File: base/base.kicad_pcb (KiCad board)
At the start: 2 copper layers, 1 part, among them U1 ESP32-WROOM-32

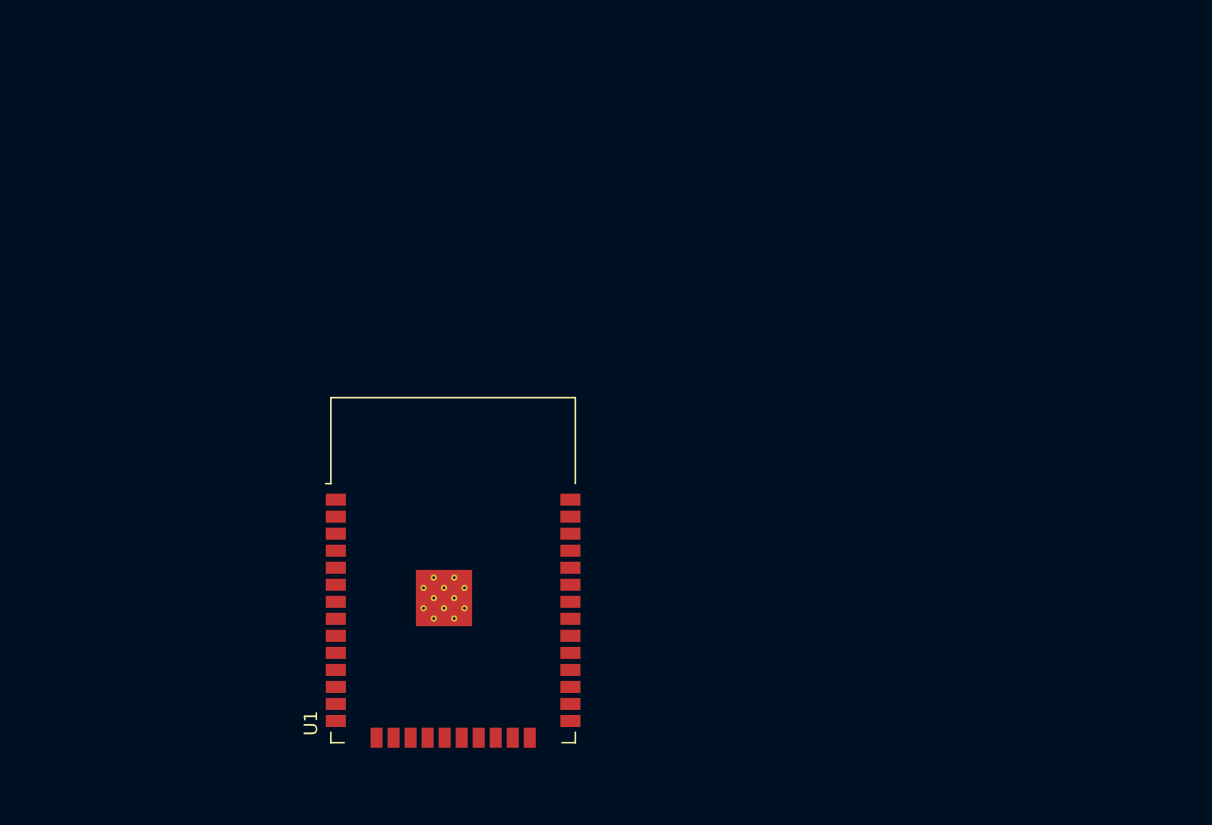
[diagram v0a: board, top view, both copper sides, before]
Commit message: add base pcb
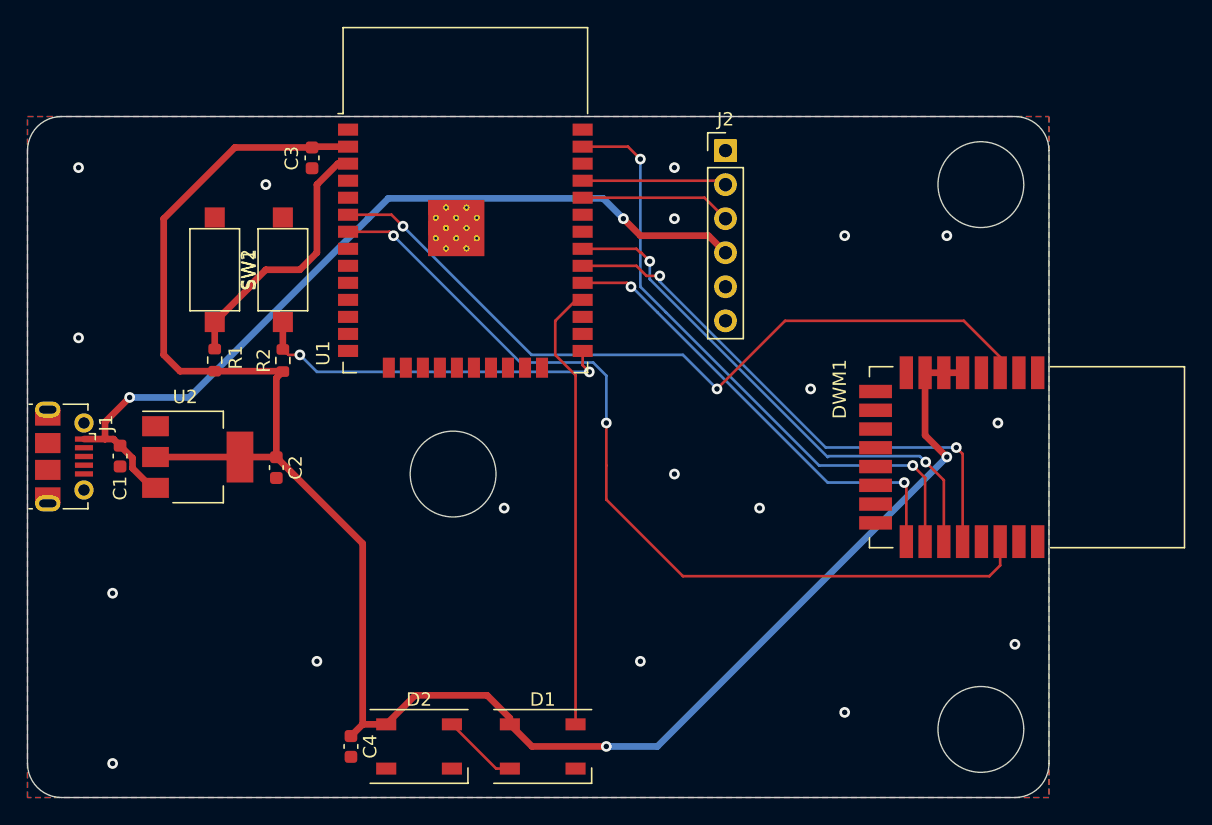
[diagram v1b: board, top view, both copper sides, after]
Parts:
- added C1: C, Capacitor_SMD:C_0603_1608Metric, F.Cu at (95.8, 88.8)
- added C2: C, Capacitor_SMD:C_0603_1608Metric, F.Cu at (107.5, 89.7)
- added C3: C, Capacitor_SMD:C_0603_1608Metric, F.Cu at (110.1, 66.6)
- added C4: C, Capacitor_SMD:C_0603_1608Metric, F.Cu at (113.0, 110.5)
- added D1: WS2812B, LED_SMD:LED_WS2812B_PLCC4_5.0x5.0mm_P3.2mm, F.Cu at (127.3, 110.5)
- added D2: WS2812B, LED_SMD:LED_WS2812B_PLCC4_5.0x5.0mm_P3.2mm, F.Cu at (118.1, 110.5)
- added DWM1: DWM1000, RF_Module:DWM1000, F.Cu at (163.5, 88.9)
- added J1: USB_B_Micro, Connector_USB:USB_Micro-B_Molex-105017-0001, F.Cu at (91.7, 88.9)
- added J2: Conn_01x06, Connector_PinHeader_2.54mm:PinHeader_1x06_P2.54mm_Vertical, F.Cu at (141.0, 66.0)
- added R1: 10K, Resistor_SMD:R_0603_1608Metric, F.Cu at (102.9, 81.7)
- added R2: 10K, Resistor_SMD:R_0603_1608Metric, F.Cu at (108.0, 81.7)
- added SW1: SW_Push_Open, Button_Switch_SMD:SW_SPST_CK_RS282G05A3, F.Cu at (102.9, 74.9)
- added SW2: SW_Push_Open, Button_Switch_SMD:SW_SPST_CK_RS282G05A3, F.Cu at (108.0, 74.9)
- added U2: LM317_SOT-223, Package_TO_SOT_SMD:SOT-223-3_TabPin2, F.Cu at (101.6, 88.9)
- moved U1 27.6 mm to (121.6, 72.7)
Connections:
- net Net-(U1-Pad1) renamed GND
- U1 pad 2: unconnected-(U1-Pad2) -> VCC
- U1 pad 25: unconnected-(U1-Pad25) -> Net-(U1-Pad25)
- U1 pad 28: unconnected-(U1-Pad28) -> WS_IN
- U1 pad 29: unconnected-(U1-Pad29) -> SS
- U1 pad 3: unconnected-(U1-Pad3) -> Net-(SW1-Pad2)
- U1 pad 30: unconnected-(U1-Pad30) -> CLK
- U1 pad 31: unconnected-(U1-Pad31) -> MISO
- U1 pad 34: unconnected-(U1-Pad34) -> ESP_RX
- U1 pad 35: unconnected-(U1-Pad35) -> ESP_TX
- U1 pad 37: unconnected-(U1-Pad37) -> MOSI
- U1 pad 6: unconnected-(U1-Pad6) -> DW_RST
- U1 pad 7: unconnected-(U1-Pad7) -> DW_IRQ
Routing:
- net VCC: track 0.00 -> 140.0 mm, vias 0 -> 2
- net DW_IRQ: track 0.00 -> 66.8 mm, vias 0 -> 2
- net 5V: track 0.00 -> 63.4 mm, vias 0 -> 2
- net DW_RST: track 0.00 -> 58.4 mm, vias 0 -> 2
- net MOSI: track 0.00 -> 46.1 mm, vias 0 -> 2
- net CLK: track 0.00 -> 40.9 mm, vias 0 -> 2
- net MISO: track 0.00 -> 39.5 mm, vias 0 -> 2
- net SS: track 0.00 -> 34.6 mm, vias 0 -> 2
- net WS_IN: track 0.00 -> 33.4 mm
- net Net-(U1-Pad25): track 0.00 -> 27.4 mm, vias 0 -> 2
- net Net-(SW1-Pad2): track 0.00 -> 19.9 mm
- net ESP_RX: track 0.00 -> 11.3 mm
- net ESP_TX: track 0.00 -> 10.8 mm
- net Net-(D1-Pad2): track 0.00 -> 5.69 mm
- net GND: vias 0 -> 18
- added copper zone on B.Cu, net GND
- added copper zone on F.Cu, net GND
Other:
- board outline added: 76.2 x 50.8 mm
